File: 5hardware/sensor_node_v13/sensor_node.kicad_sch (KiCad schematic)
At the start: 38 parts, among them J1 Conn_01x08_Socket, J2 Conn_01x08_Socket, Q2 AO3401A, Q3 MMBT5551L, Q4 AO3401A, SW1 SW_Push, SW2 SW_Push, SW3 SW_Push, SW4 SW_Reed, SW5 SW_Push, SW6 SW_Push, SW7 SW_Push, U1 ESP-12F, U12 APDS-9960, U13 SHT31-DIS, U17 BH1750FVI-TR, U2 2N7002DW, U7 XC6206PxxxMR, U8 TPL5110

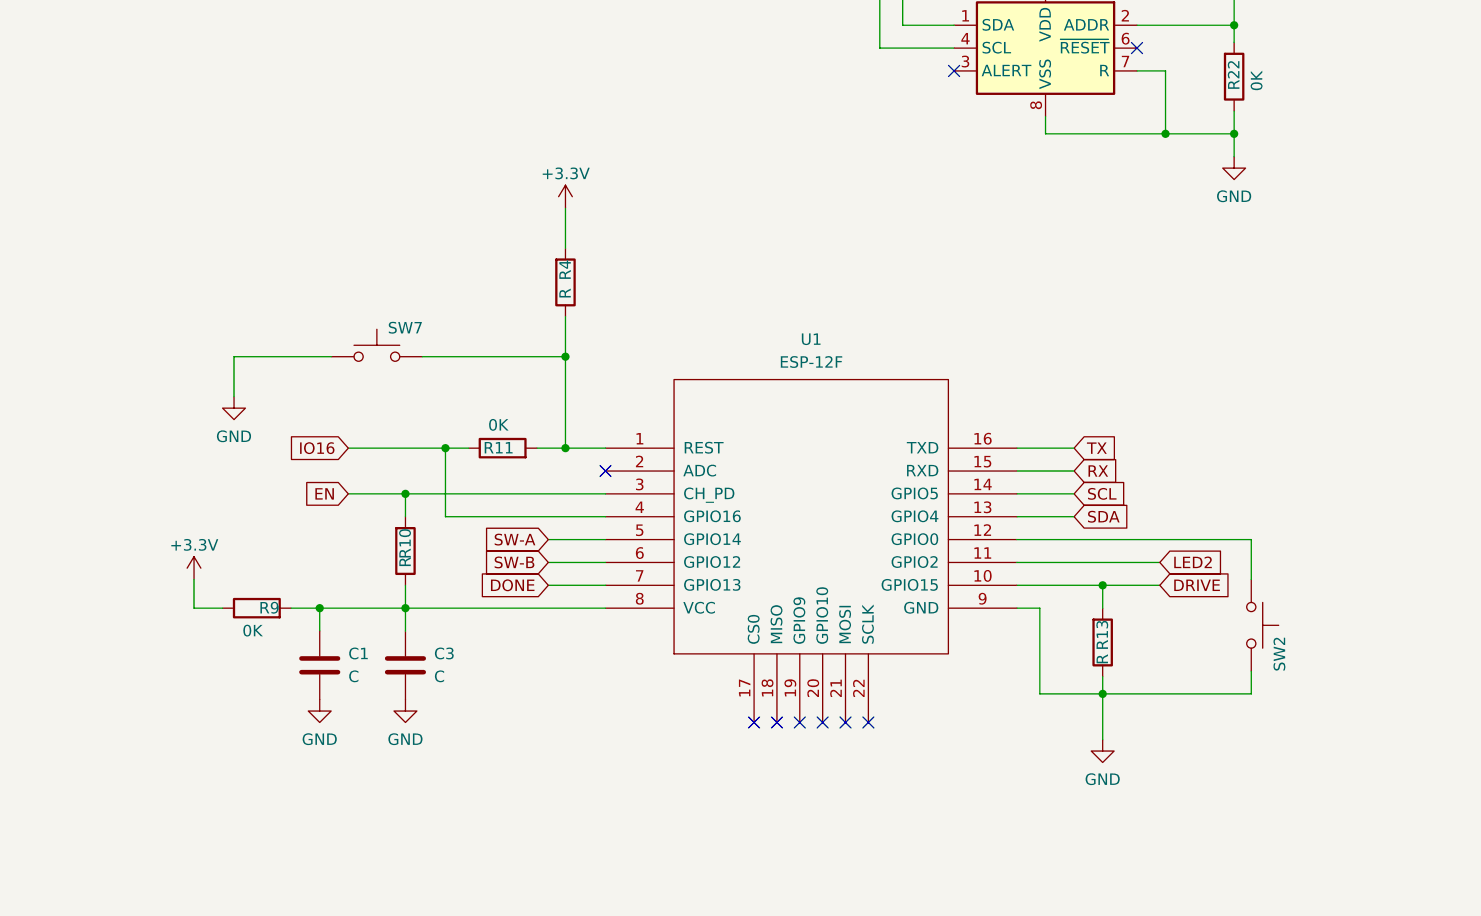
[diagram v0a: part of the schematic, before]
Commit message: cleanup.
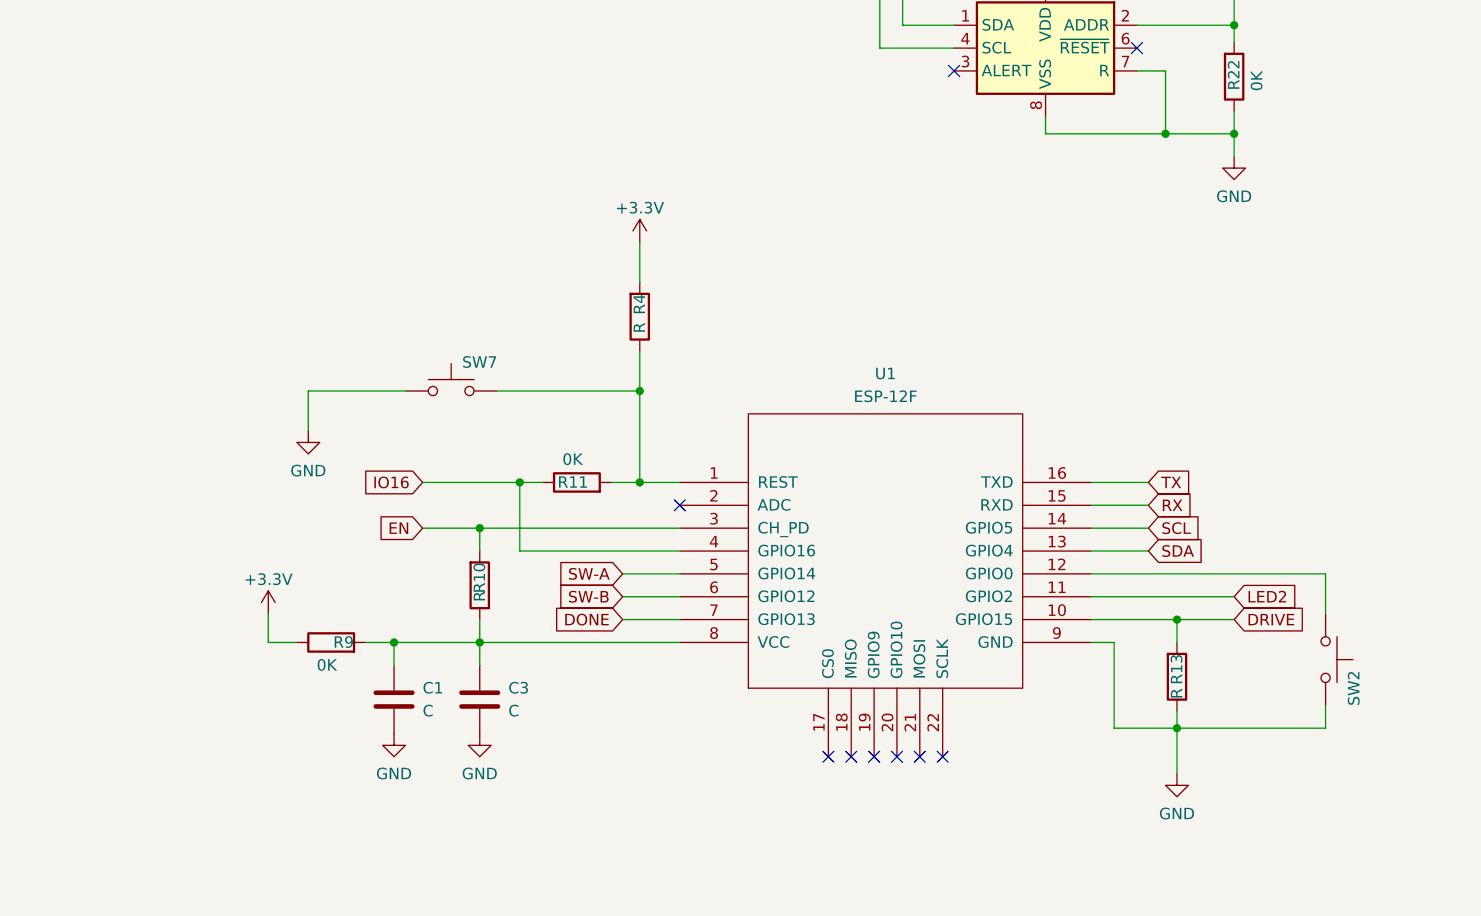
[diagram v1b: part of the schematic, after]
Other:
- moved on the sheet: C1, C3, R10, R11, R13, R4, R9, SW2, SW7, U1
